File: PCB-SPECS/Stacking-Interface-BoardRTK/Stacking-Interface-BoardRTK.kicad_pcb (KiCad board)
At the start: 2 copper layers, 65 x 83 mm, 15 parts

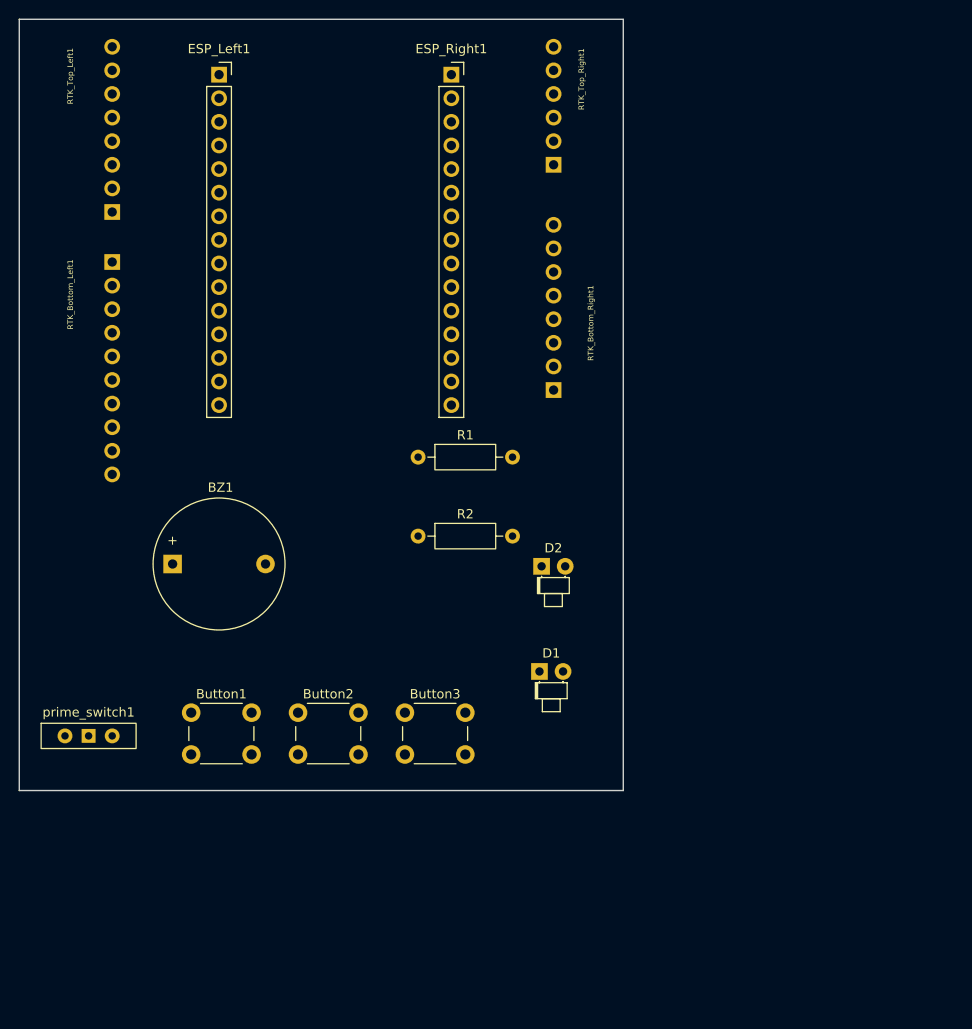
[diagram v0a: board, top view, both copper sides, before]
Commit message: finished designing pcb
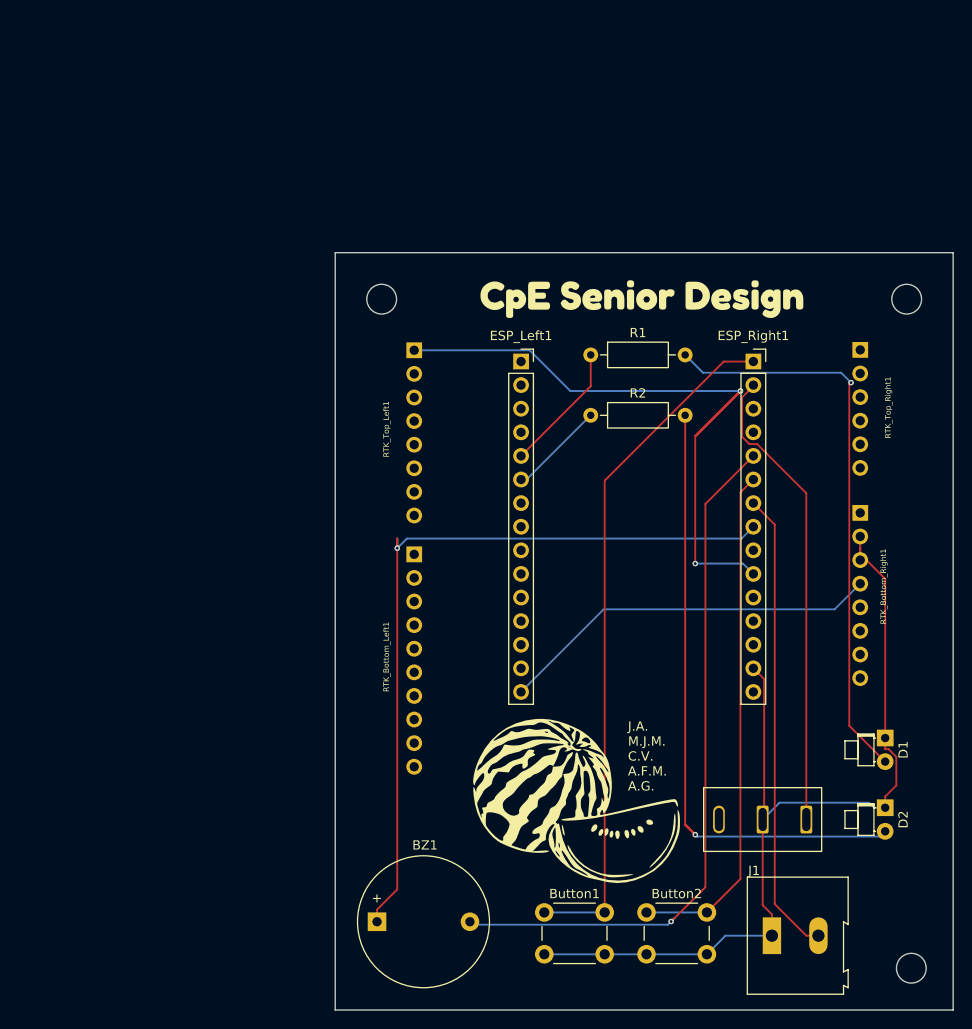
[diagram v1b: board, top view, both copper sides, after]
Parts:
- removed Button3: SW_Push, Button_Switch_THT:SW_PUSH_6mm
- added G***: LOGO, graphics:watermelon, F.Cu at (117.0, 108.0)
- added J1: Screw_Terminal_01x02, TerminalBlock:TerminalBlock_Altech_AK300-2_P5.00mm, F.Cu at (138.0, 122.5)
- added hole1: MountingHole_3.2mm_M3, MountingHole:MountingHole_3.2mm_M3, F.Cu at (96.0, 54.0)
- added hole2: MountingHole_3.2mm_M3, MountingHole:MountingHole_3.2mm_M3, F.Cu at (152.5, 54.0)
- added hole3: MountingHole_3.2mm_M3, MountingHole:MountingHole_3.2mm_M3, F.Cu at (153.0, 126.0)
- added kibuzzard-69A9F479: G***, kibuzzard-69A9F479, F.Cu at (124.0, 54.0)
- prime_switch1: footprint Button_Switch_THT:SW_Slide-03_Wuerth-WS-SLTV_10x2.5x6.4_P2.54mm -> watermelonstuff:spdt_switch
- moved prime_switch1 73.1 mm to (137.0, 110.0)
- moved RTK_Bottom_Left1 45.2 mm to (99.5, 81.5)
- moved D2 45.2 mm to (150.2, 108.7), turned to -90 degrees
- moved ESP_Left1 44.8 mm to (111.0, 60.7)
- moved ESP_Right1 44.8 mm to (136.0, 60.7)
- moved BZ1 44.3 mm to (95.5, 121.0)
- moved Button1 43.7 mm to (113.5, 120.0)
- moved Button2 43.2 mm to (124.5, 120.0)
- moved RTK_Top_Right1 38.5 mm to (147.5, 59.5), turned to 180 degrees
- moved D1 37.9 mm to (150.2, 101.2), turned to -90 degrees
- moved RTK_Top_Left1 35.7 mm to (99.5, 59.5), turned to 180 degrees
- moved RTK_Bottom_Right1 35.5 mm to (147.5, 77.0), turned to 180 degrees
- moved R2 22.7 mm to (118.5, 66.5)
- moved R1 21.6 mm to (118.5, 60.0)
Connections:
- ESP_Left1 pad 15: unconnected-(ESP_Left1-Pin_15-Pad15) -> VCC
- RTK_Bottom_Right1 pad 1: GND -> unconnected-(RTK_Bottom_Right1-Pin_1-Pad1)
- RTK_Bottom_Right1 pad 3: unconnected-(RTK_Bottom_Right1-Pin_3-Pad3) -> GND
- RTK_Bottom_Right1 pad 4: unconnected-(RTK_Bottom_Right1-Pin_4-Pad4) -> VCC
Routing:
- net GND: track 0.00 -> 102.0 mm
- net Net-(ESP_Right1-Pin_10): track 0.00 -> 91.8 mm, vias 0 -> 2
- net Net-(BZ1-+): track 0.00 -> 84.6 mm, vias 0 -> 1
- net Net-(BZ1--): track 0.00 -> 76.7 mm, vias 0 -> 1
- net Net-(ESP_Right1-Pin_1): track 0.00 -> 74.3 mm
- net Net-(D2-A): track 0.00 -> 72.5 mm, vias 0 -> 1
- net Net-(D1-A): track 0.00 -> 61.6 mm, vias 0 -> 1
- net Net-(ESP_Right1-Pin_6): track 0.00 -> 55.2 mm
- net Net-(ESP_Right1-Pin_2): track 0.00 -> 50.6 mm
- net Net-(ESP_Right1-Pin_7): track 0.00 -> 50.2 mm
- net VCC: track 0.00 -> 41.3 mm
- net Net-(ESP_Left1-Pin_5): track 0.00 -> 14.0 mm
- net Net-(ESP_Left1-Pin_6): track 0.00 -> 10.4 mm
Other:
- board size 65 x 83 mm -> 66.5 x 81.5 mm
- board text added: "03/05/2026"
- board text added: "Garden E-Cutters: Mid Layer PCB"
- board text added: "J.A. M.J.M. C.V. A.F.M. A.G."
